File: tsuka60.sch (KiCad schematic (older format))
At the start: 165 parts, among them SW1 SW_Push, U1 ATmega32U4-AU, Y1 Resonator_Small

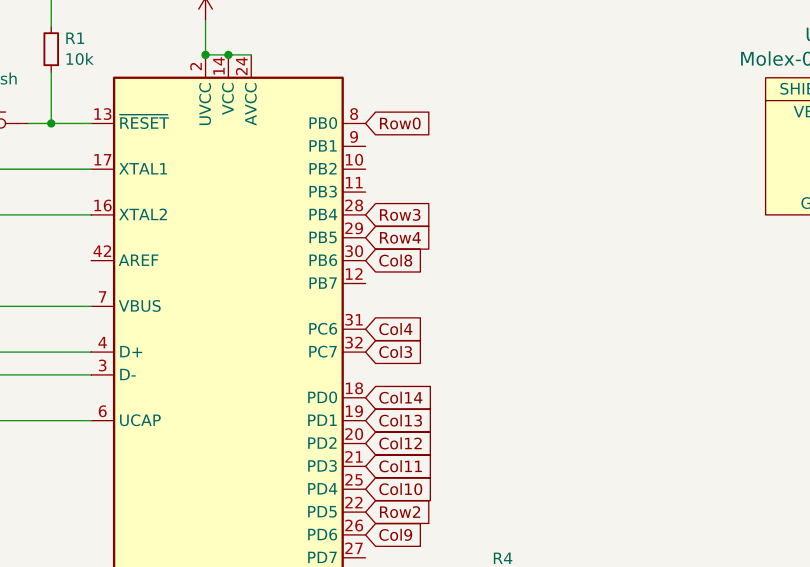
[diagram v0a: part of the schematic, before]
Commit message: completed all traces
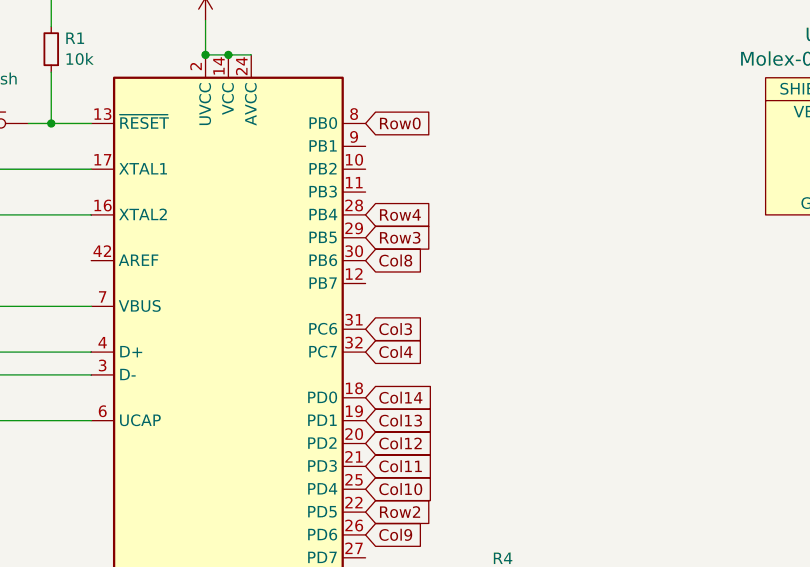
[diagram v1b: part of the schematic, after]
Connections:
- net Col3: now also U1.31 (PC6); no longer U1.32 (PC7)
- net Col4: now also U1.32 (PC7); no longer U1.31 (PC6)
- net Row3: now also U1.29 (PB5); no longer U1.28 (PB4)
- net Row4: now also U1.28 (PB4); no longer U1.29 (PB5)
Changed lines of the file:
@@
 Text GLabel 5750 12050 2    50   Input ~ 0
 Row2
+Text GLabel 5750 10850 2    50   Input ~ 0
+Row3
 Text GLabel 5750 10750 2    50   Input ~ 0
-Row3
-Text GLabel 5750 10850 2    50   Input ~ 0
 Row4
 Text GLabel 5750 12750 2    50   Input ~ 0
@@
 Text GLabel 5750 12950 2    50   Input ~ 0
 Col2
+Text GLabel 5750 11250 2    50   Input ~ 0
+Col3
 Text GLabel 5750 11350 2    50   Input ~ 0
-Col3
-Text GLabel 5750 11250 2    50   Input ~ 0
 Col4
 Text GLabel 5750 13250 2    50   Input ~ 0
